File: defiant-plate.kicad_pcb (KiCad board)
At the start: 2 copper layers, 126.1 x 99.6 mm, 28 parts, among them T0 SW_PUSH, T1 SW_PUSH, T2 SW_PUSH, T3 SW_PUSH, T4 SW_PUSH

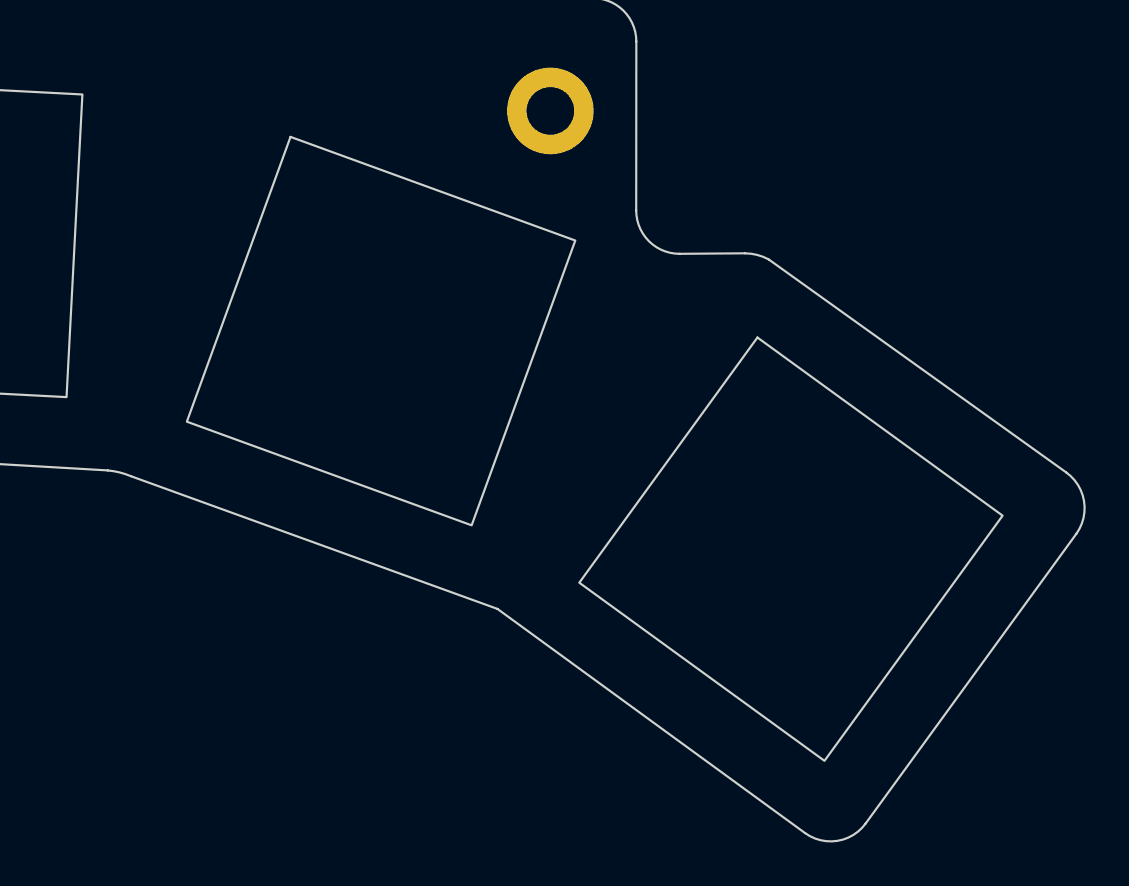
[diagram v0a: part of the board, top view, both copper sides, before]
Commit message: Experimental: Tighten thumb key placing
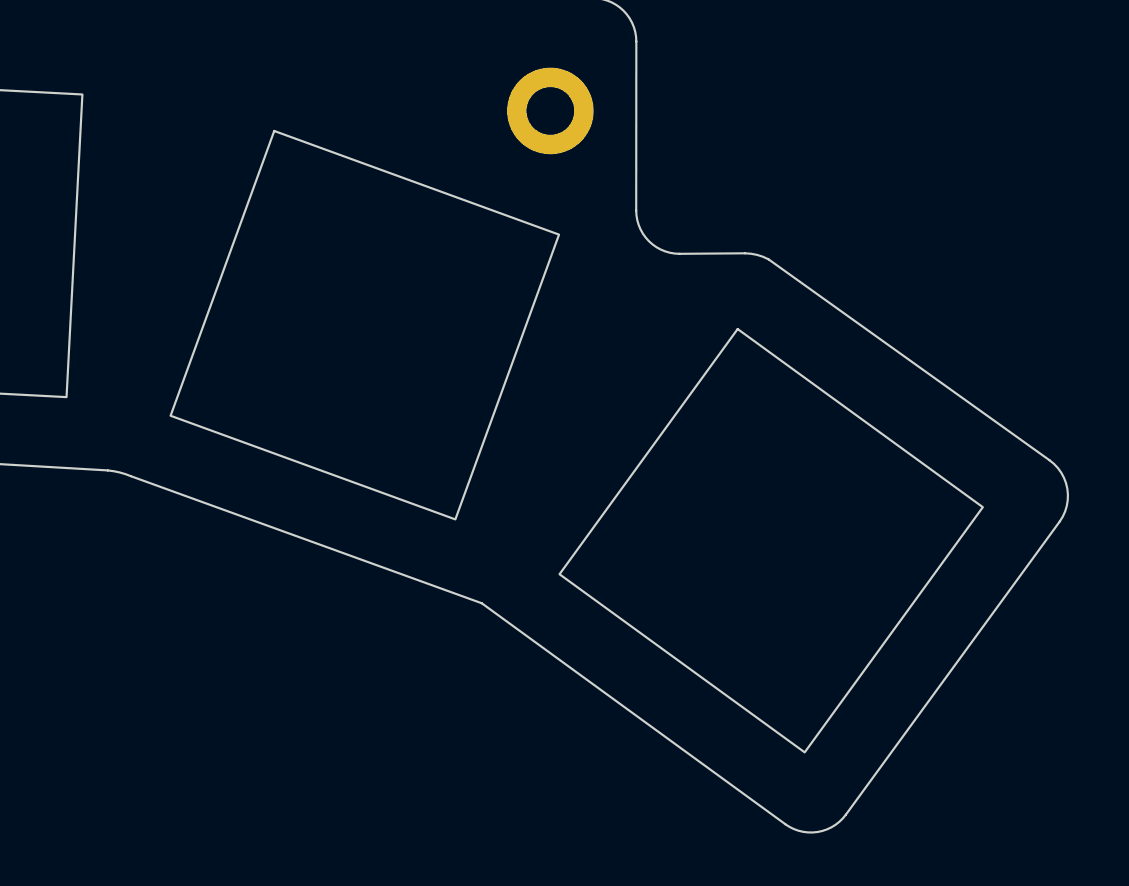
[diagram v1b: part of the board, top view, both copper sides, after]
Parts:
- moved T4 0.99 mm to (191.4, 133.6)
- moved T3 0.80 mm to (172.6, 123.6)
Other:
- board size 126.1 x 99.6 mm -> 125.4 x 99.2 mm
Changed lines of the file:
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@@
   )
   (footprint "Defiant:SW_Gateron_LowProfile_Plate" (layer "F.Cu")
-    (at 192.333168 133.954069 -36)
+    (at 191.41961 133.562895 -36)
     (descr "Gateron Low Profile (KS-27 & KS-33) style mechanical keyboard switch, Gateron Low Profile hot-swap socket and through-hole soldering, the hole of the socket is plated, single-sided mounting. Gateron Low Profile and Cherry MX Low Profile are NOT compatible.")
     (tags "switch, low_profile, hot_swap")
@@
   )
   (footprint "Defiant:SW_Gateron_LowProfile_Plate" (layer "F.Cu")
-    (at 173.398584 123.880307 -20)
+    (at 172.64683 123.606691 -20)
     (descr "Gateron Low Profile (KS-27 & KS-33) style mechanical keyboard switch, Gateron Low Profile hot-swap socket and through-hole soldering, the hole of the socket is plated, single-sided mounting. Gateron Low Profile and Cherry MX Low Profile are NOT compatible.")
     (tags "switch, low_profile, hot_swap")
@@
   (gr_arc (start 174.264362 51.813324) (mid 175.678568 52.399114) (end 176.264362 53.813324)
     (stroke (width 0.1) (type default)) (layer "Edge.Cuts"))
-  (gr_line (start 161.844251 130.583323) (end 178.774251 136.713323)
+  (gr_line (start 161.844251 130.583323) (end 178.052037 136.45323)
     (stroke (width 0.1) (type default)) (layer "Edge.Cuts"))
   (gr_arc (start 160.771011 130.315765) (mid 161.317896 130.408369) (end 161.844251 130.583323)
@@
   (gr_line (start 143.384251 129.303322) (end 160.771011 130.315765)
     (stroke (width 0.1) (type default)) (layer "Edge.Cuts"))
-  (gr_arc (start 205.046042 130.406818) (mid 205.870563 131.722611) (end 205.523182 133.236042)
+  (gr_arc (start 204.275479 129.844207) (mid 205.1 131.16) (end 204.752619 132.673431)
     (stroke (width 0.1) (type default)) (layer "Edge.Cuts"))
   (gr_arc (start 195.269951 98.659951) (mid 194.684179 100.074179) (end 193.269951 100.659951)
@@
   (gr_line (start 193.27 100.65) (end 175.85 100.65)
     (stroke (width 0.1) (type default)) (layer "Edge.Cuts"))
-  (gr_line (start 205.046042 130.406818) (end 191.296753 120.563385)
+  (gr_line (start 204.275479 129.844207) (end 191.296753 120.563385)
     (stroke (width 0.1) (type default)) (layer "Edge.Cuts"))
   (gr_line (start 98.774252 53.813324) (end 98.774251 59.813323)
@@
   (gr_arc (start 98.774252 53.813324) (mid 99.360038 52.39911) (end 100.774252 51.813324)
     (stroke (width 0.1) (type default)) (layer "Edge.Cuts"))
-  (gr_arc (start 195.782279 146.628903) (mid 194.477115 147.428701) (end 192.988674 147.071366)
+  (gr_arc (start 194.870117 146.218857) (mid 193.564943 147.018681) (end 192.076512 146.66132)
     (stroke (width 0.1) (type default)) (layer "Edge.Cuts"))
   (gr_line (start 79.774251 61.813323) (end 79.774251 116.303323)
@@
   (gr_line (start 100.774252 129.303322) (end 143.384251 129.303322)
     (stroke (width 0.1) (type default)) (layer "Edge.Cuts"))
-  (gr_line (start 205.523182 133.236042) (end 195.782279 146.628903)
+  (gr_line (start 204.752619 132.673431) (end 194.870116 146.218833)
     (stroke (width 0.1) (type default)) (layer "Edge.Cuts"))
   (gr_line (start 190.210153 120.286479) (end 187.184214 120.31)
@@
   (gr_line (start 193.26427 61.203304) (end 176.264251 61.203304)
     (stroke (width 0.1) (type default)) (layer "Edge.Cuts"))
-  (gr_line (start 192.988674 147.071366) (end 178.774251 136.713323)
+  (gr_line (start 192.076512 146.66132) (end 178.052037 136.45323)
     (stroke (width 0.1) (type default)) (layer "Edge.Cuts"))
   (gr_arc (start 187.184214 120.31) (mid 185.77 119.724214) (end 185.184214 118.31)
@@
     (effects (font (size 1 1) (thickness 0.15)) (justify left bottom))
   )
+  (group "" (id 80c8c62c-9fcb-4d36-b24e-8b415d0671ae)
+    (members
+      00bf3f3e-b9d5-4964-8f21-674bc8874993
+      04572bb3-2238-4247-a8dd-3b13a789e49b
+      0fcea472-68b1-44c8-ac8d-77b0d9fa2038
+      137e6e71-51f5-490b-bcf5-38d57dbf122b
+      187880dd-dbe2-4f07-9fd4-3625e335b4af
+      1b6d2ddd-5e23-4b2f-8eb2-bbd8625d822b
+      1d862835-9a83-44e9-a4a0-118baa66f62e
+      26d3e322-20e0-4678-9fe2-7c2475af3b05
+      2907f11e-160f-4618-beb6-c4b8d875aff3
+      2ef10bcc-73e2-461e-97c1-eefc00f460ea
+      2f57fc79-a697-4788-95e9-1dab930f9fe4
+      3ecf6329-27cf-47be-9343-7aa17994766d
+      3f0822e6-73b7-49f4-bac1-605b2b248c26
+      41e2dbde-a439-40e1-bcd7-f6f599d7119c
+      42b800f3-1d83-4b55-9aad-cf2cad6d1635
+      50627230-a6c5-43fa-b095-e8d76ef6b16c
+      54d0a574-9f7d-4f7c-8c64-fdc0ca3e3258
+      57ea1219-470e-4400-b2e9-9a4d3fa6eb14
+      657e030a-431b-4145-aabd-bbb684768414
+      66c119ba-26b8-4680-b1a1-a54c32bab990
+      6d22f171-ca04-4436-bead-2aa30f1570a9
+      6f5c9bba-3061-40f5-9d11-c229c1d8b13d
+      82f5b0c4-158c-4037-ae77-8f41119a89a5
+      8d36f90a-d68c-4fa8-bdc4-4bb3faac0c2a
+      8ecc577c-01b8-442f-871c-9ae66f177b6b
+      9ceb8403-4be3-4063-8ecc-b1eaea6e793f
+      a6f6d37f-4fc6-4f31-8d9c-a2c1cc73ed61
+      ab194198-a741-481c-b59c-6c8ed288259b
+      ab233530-da3c-4273-8376-32f9629841c1
+      ab395b4b-0ee3-464b-be4b-27ac47187c30
+      b4fc6401-e446-4953-a472-ebde5c8b8d66
+      bb08e371-c793-4f6c-bc66-a24afb154a1f
+      c0b919f3-b047-4cb3-8561-e3c8630304c2
+      d211463e-9430-423f-89b0-754f99027c05
+      d90c28dc-664c-46a6-b702-f5e37777b307
+      d9f6b089-a5d5-4ed1-938c-463d85a0e7a5
+      da04bc08-2770-4f4c-a7d2-85dfcb33a628
+      ea6f10e5-2714-4943-8970-3adfed318d99
+      f9c48685-cabf-4918-b0c4-b06fd2c1c7a6
+    )
+  )
 )
